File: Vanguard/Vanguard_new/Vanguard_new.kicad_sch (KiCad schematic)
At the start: 0 parts

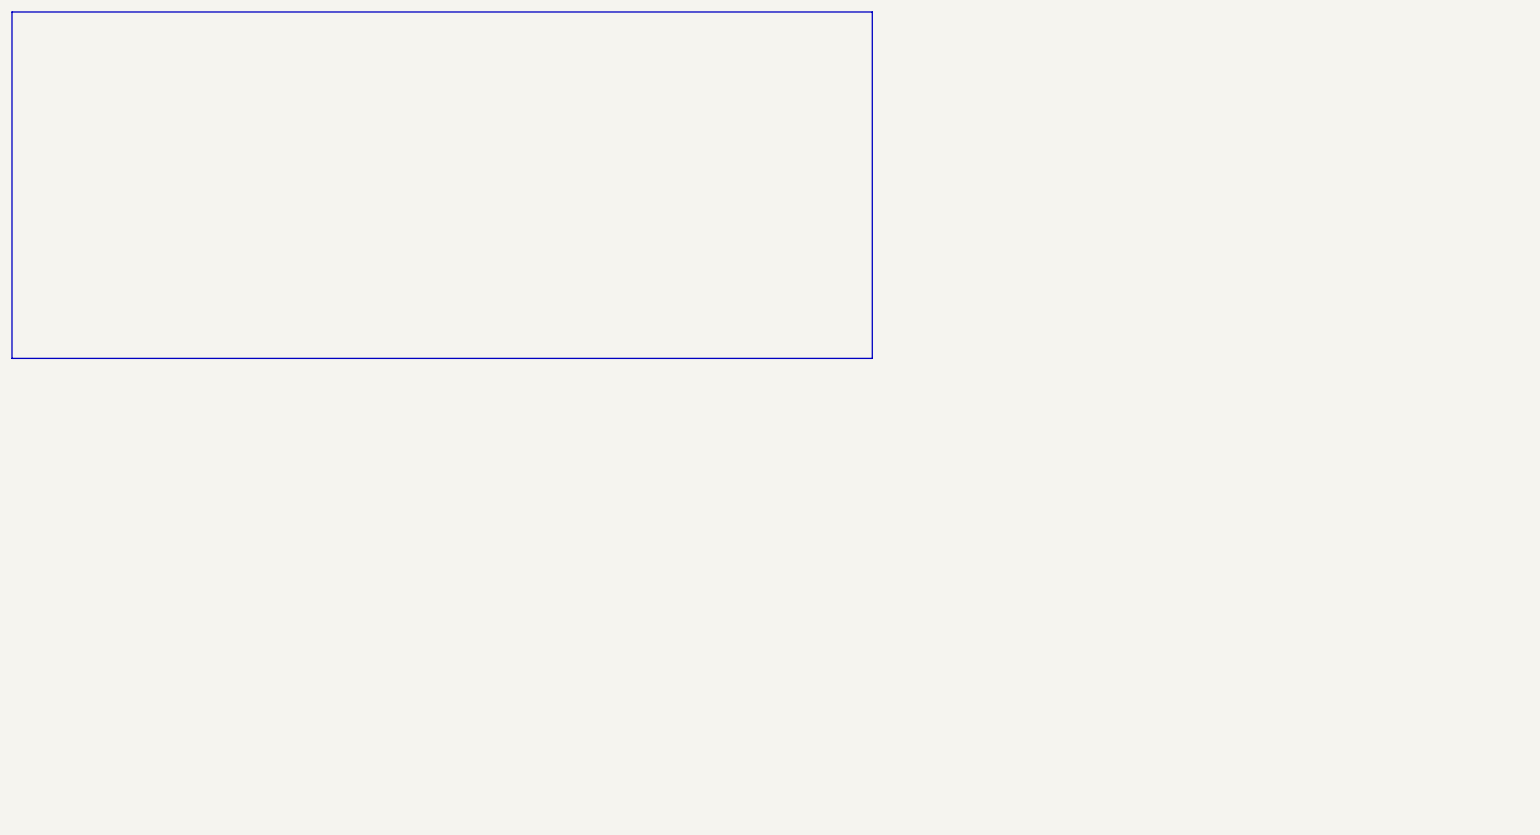
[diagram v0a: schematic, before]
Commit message: opened a new schematic
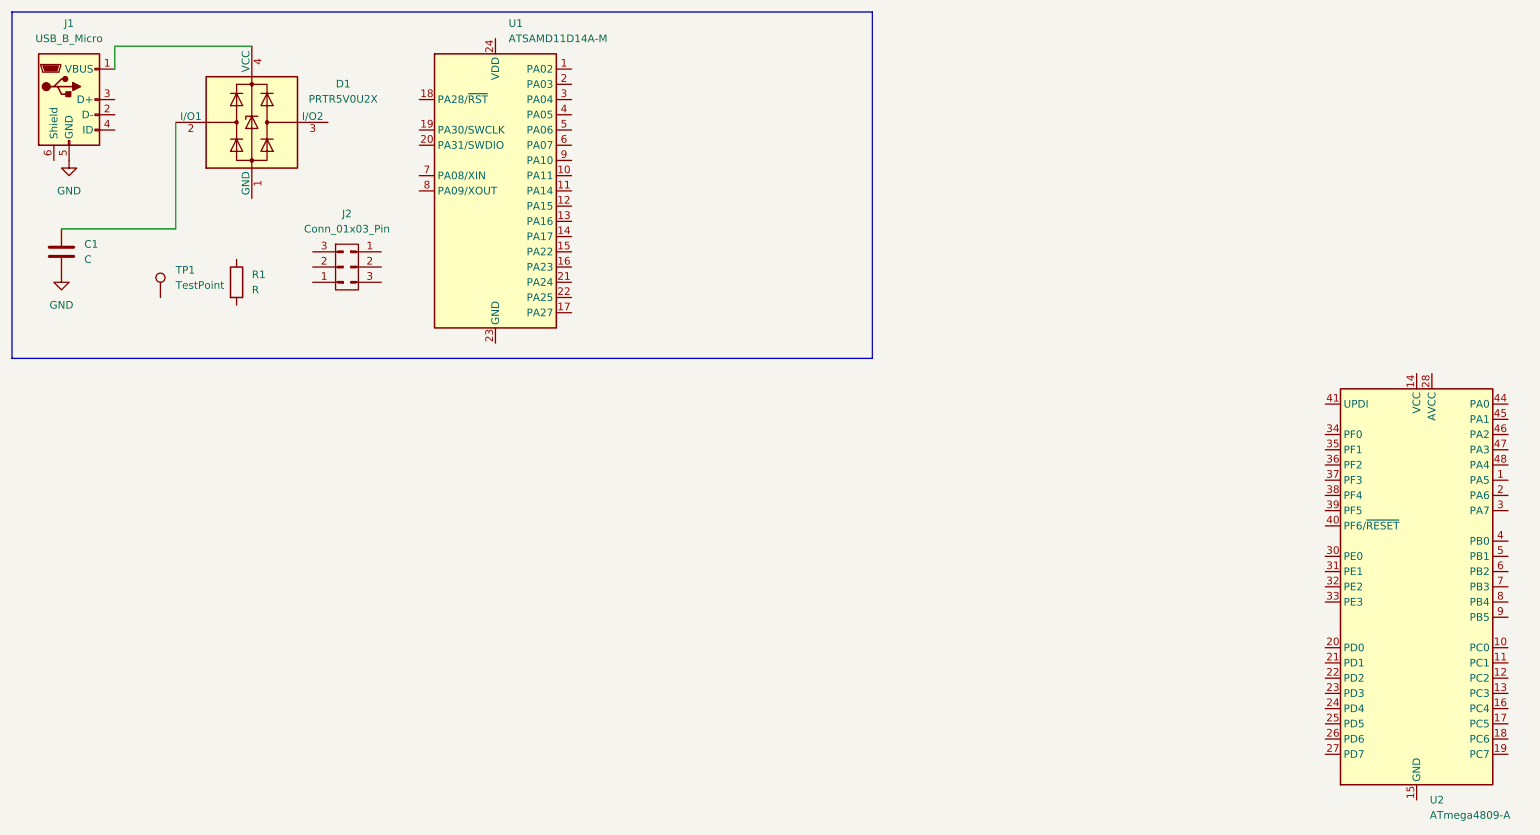
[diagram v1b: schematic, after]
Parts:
- added C1: C, symbol Device:C
- added D1: PRTR5V0U2X, Package_TO_SOT_SMD:SOT-143, symbol Power_Protection:PRTR5V0U2X
- added J1: USB_B_Micro, symbol Connector:USB_B_Micro
- added J2: Conn_01x03_Pin, symbol Connector:Conn_01x03_Pin
- added R1: R, symbol Device:R
- added TP1: TestPoint, symbol Connector:TestPoint
- added U1: ATSAMD11D14A-M, Package_DFN_QFN:QFN-24-1EP_4x4mm_P0.5mm_EP2.6x2.6mm, symbol MCU_Microchip_SAMD:ATSAMD11D14A-M
- added U2: ATmega4809-A, Package_QFP:TQFP-48_7x7mm_P0.5mm, symbol MCU_Microchip_ATmega:ATmega4809-A
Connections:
- new net: C1.1, D1.2 (I/O1)
- new net: D1.4 (VCC), J1.1 (VBUS)
- new net: U2.14 (VCC), U2.42 (VCC)
- new net: U2.15 (GND), U2.29 (GND), U2.43 (GND)
- new net GND: C1.2, J1.5 (GND)
